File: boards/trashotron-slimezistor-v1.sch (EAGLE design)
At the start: 17 parts, among them IC1 2967-MP6500, IC2 2967-MP6500, IC3 2967-MP6500, J4 455-1750-1-ND, J6 455-1750-1-ND, J9 455-1750-1-ND, U2 LM358

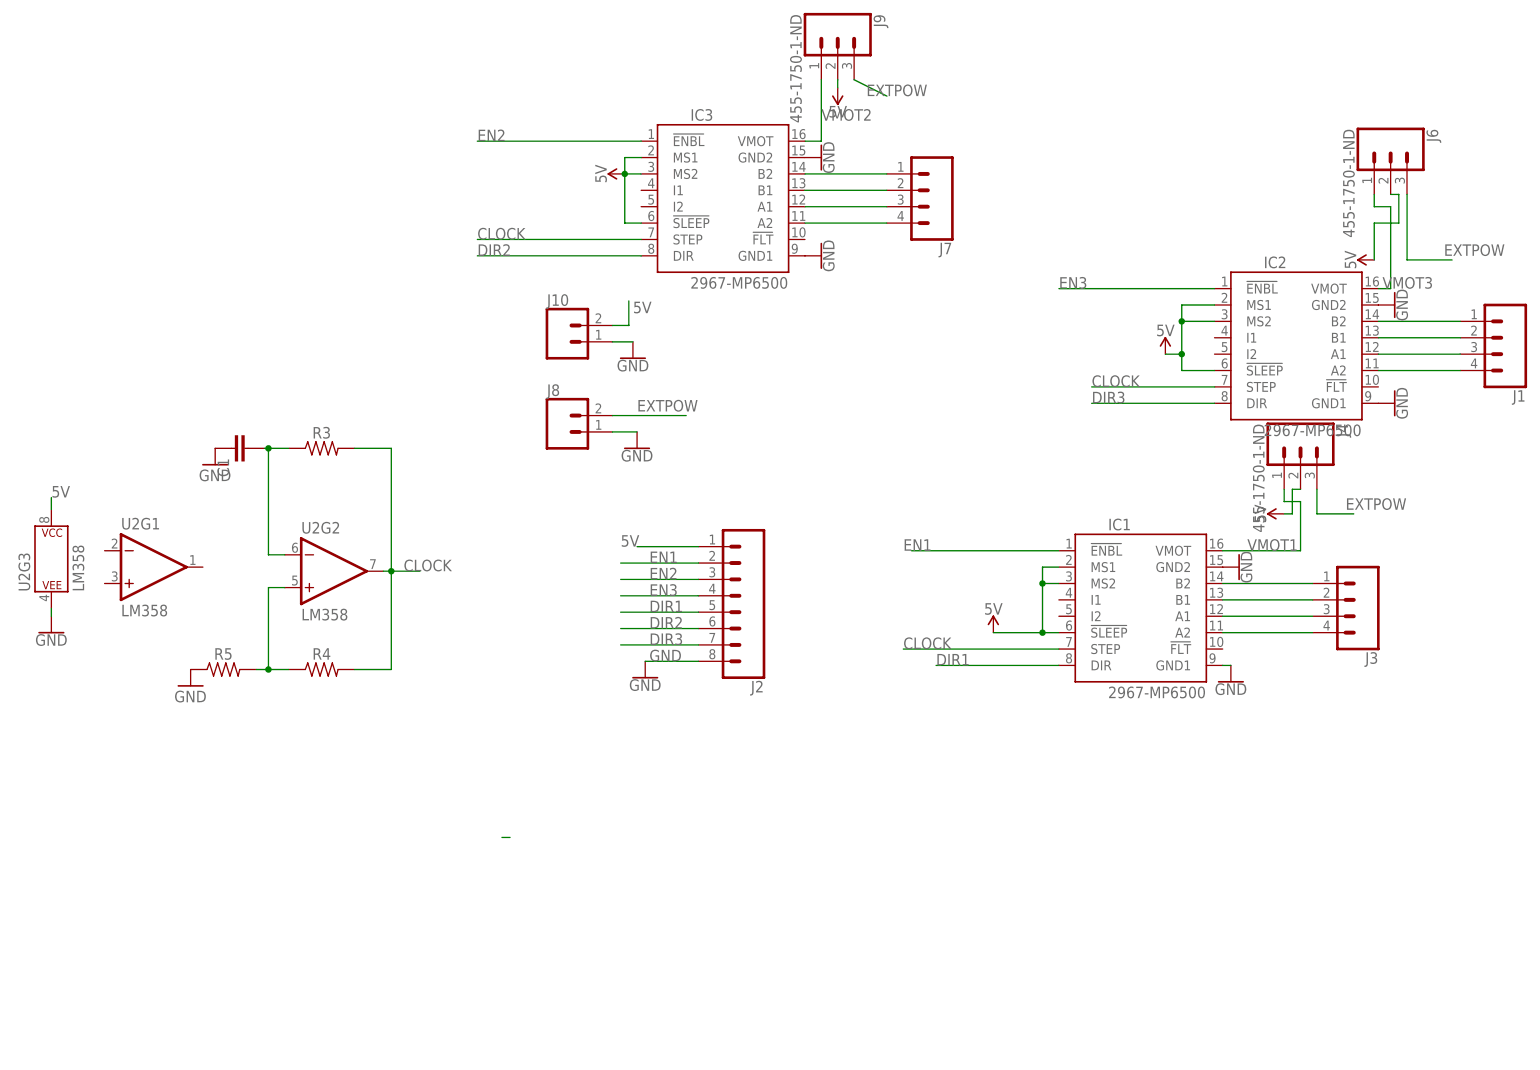
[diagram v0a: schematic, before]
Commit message: lots of work on pcb layout
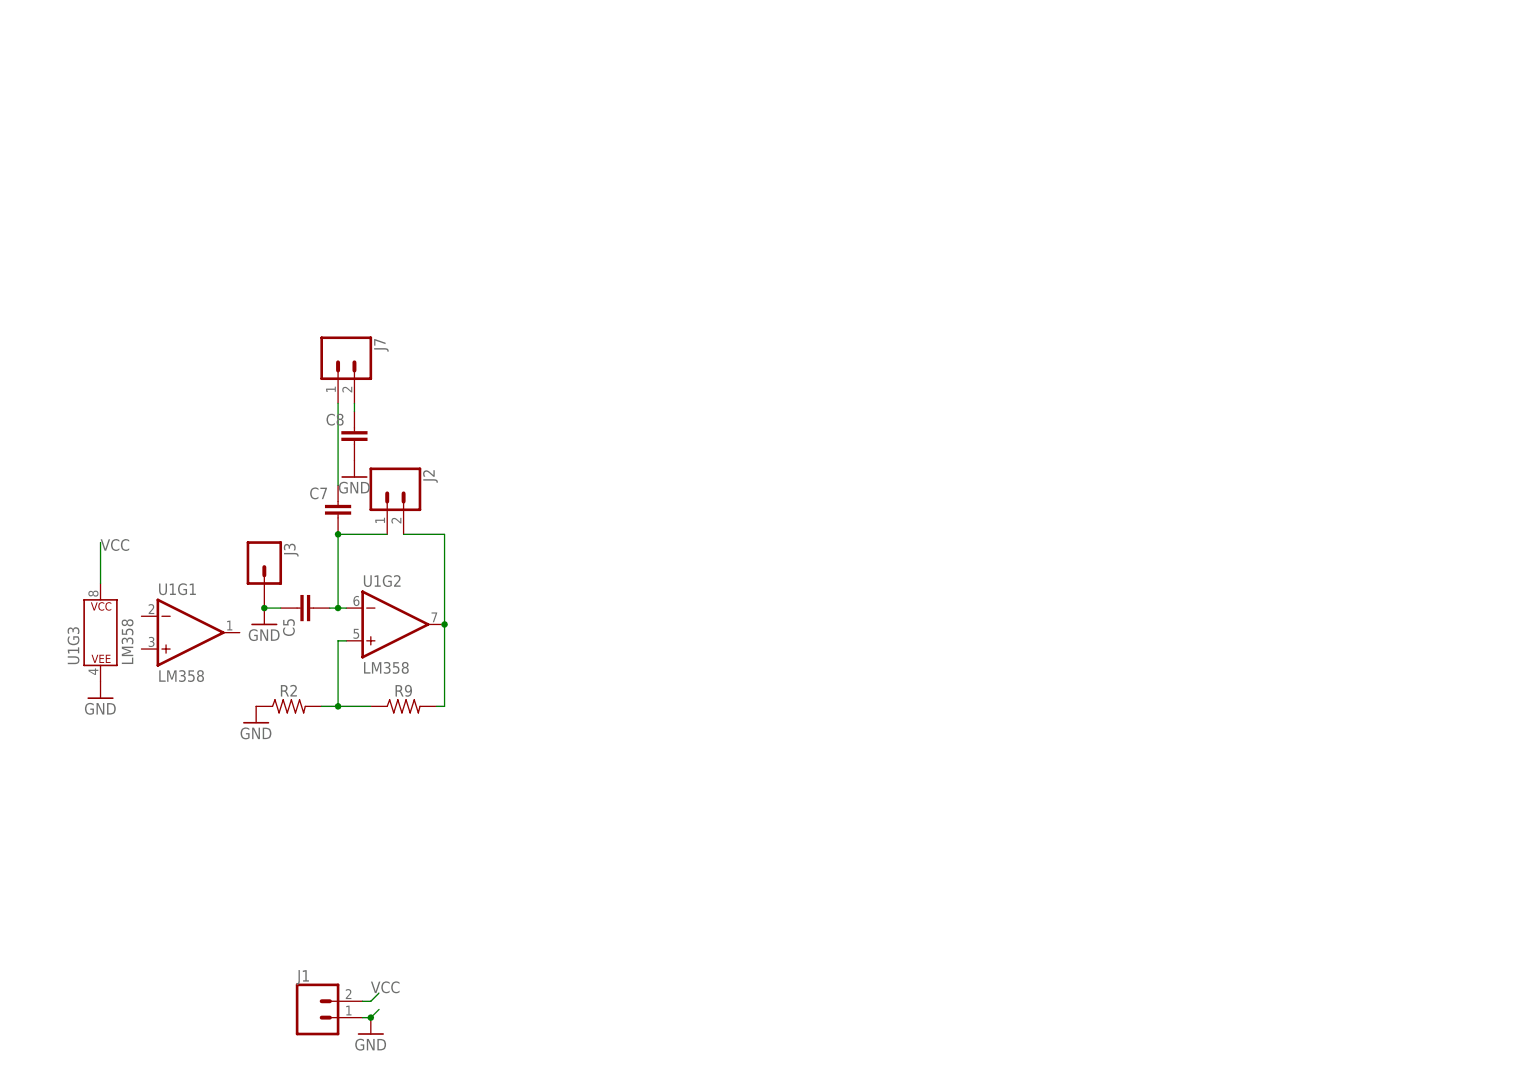
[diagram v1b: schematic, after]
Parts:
- removed C1: (no value), rcl:C-EU050-050X075
- removed IC1, IC2, IC3: 2967-MP6500, pololu-stepper-driver:2967-MP6500
- removed J10, J8: (no value), SparkFun-Connectors:CONN_02
- removed J4, J6, J9: 455-1750-1-ND, SparkFun-Connectors:CONN_03
- removed R3, R4, R5: (no value), SparkFun-Resistors:RESISTORAXIAL-0.3
- removed U2: LM358, SparkFun-IC-Amplifiers:LM358
- added C5, C7, C8: (no value), rcl:C-EU050-050X075
- added R2, R9: (no value), SparkFun-Resistors:RESISTORAXIAL-0.3
- added U1: LM358, SparkFun-IC-Amplifiers:LM358
- J1, J7: device SparkFun-Connectors:CONN_04 -> SparkFun-Connectors:CONN_02
- J2: device SparkFun-Connectors:CONN_08" -> SparkFun-Connectors:CONN_02
- J3: device SparkFun-Connectors:CONN_04 -> SparkFun-Connectors:CONN_01
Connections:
- removed net 5V: IC1.!SLEEP, IC1.MS1, IC1.MS2, IC2.!SLEEP, IC2.MS1, IC2.MS2, IC3.!SLEEP, IC3.MS1, IC3.MS2, J10.2, J2.1, J4.2, J6.2, J9.2, U2G3.P$V+
- removed net CLOCK: IC1.STEP, IC2.STEP, IC3.STEP, R3.2, R4.2, U2G2.OUT
- removed net DIR1: IC1.DIR, J2.5
- removed net DIR2: IC3.DIR, J2.6
- removed net DIR3: IC2.DIR, J2.7
- removed net EN1: IC1.!ENBL, J2.2
- removed net EN2: IC3.!ENBL, J2.3
- removed net EN3: IC2.!ENBL, J2.4
- removed net EXTPOW: J4.3, J6.3, J8.2, J9.3
- removed net N$1: IC3.B2, J7.1
- removed net N$11: IC2.A1, J1.3
- removed net N$13: IC3.A1, J7.3
- removed net N$18: C1.2, R3.1, U2G2.-IN
- removed net N$19: R4.1, R5.2, U2G2.+IN
- removed net N$4: IC3.B1, J7.2
- removed net N$6: IC1.B1, J3.2
- removed net N$7: IC1.A1, J3.3
- removed net N$8: IC1.A2, J3.4
- removed net N$9: IC2.B2, J1.1
- removed net VMOT1: IC1.VMOT, J4.1
- removed net VMOT2: IC3.VMOT, J9.1
- removed net VMOT3: IC2.VMOT, J6.1
- new net N$16: C7.1, J7.1
- new net VCC: J1.2, U1G3.P$V+
- net GND: now also C5.1, C8.2, J1.1, J3.1, R2.1, U1G3.P$V-; no longer C1.1, IC1.GND1, IC1.GND2, IC2.GND1, IC2.GND2, IC3.GND1, IC3.GND2, J10.1, J2.8, J8.1, R5.1, U2G3.P$V-
- net N$10: now also R2.2, R9.1, U1G2.+IN; no longer IC2.B1, J1.2
- net N$12: now also C5.2, C7.2, J2.1, U1G2.-IN; no longer IC2.A2, J1.4
- net N$14: now also C8.1, J7.2; no longer IC3.A2, J7.4
- net N$5: now also J2.2, R9.2, U1G2.OUT; no longer IC1.B2, J3.1
